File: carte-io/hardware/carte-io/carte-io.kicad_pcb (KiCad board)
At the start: 4 copper layers, 117.5 x 88.5 mm, 193 parts, among them J1 USB_C_Receptacle_USB2.0_14P, J10 JST_PH_B4B, J11 JST_PH_B4B, J12 JST_PH_B4B, J13 JST_PH_B4B, J14 JST_PH_B4B, J15 JST_PH_B4B, J16 JST_PH_B4B, J17 JST_PH_B4B, J18 JST_PH_B4B, J19 JST_PH_B4B, J2 JST-XH_S2B-XH-A, J20 Conn_02x08_Odd_Even, J22 JST_PH_B6B, J23 JST_PH_B4B, J24 JST_PH_B4B, J25 JST_PH_B4B, J26 JST-PH-B2B, J27 JST_PH_B5B, J3 FTSH-105-01-L-DV-007, J4 JST_PH_B4B, J5 JST_PH_B4B, J6 JST_PH_B4B, J7 JST_PH_B4B, J8 TSW-104-07-G-T, J9 TSW-104-07-G-T, SW1 SW_Push, SW2 SW_Push, U1 STM32U545VETx, U10 CM1293A-04SO, U11 74LVC125APW, U12 LSM6DS3, U13 LIS2MDL, U14 LPS22DF, U15 PCA9544APW, U16 LT1963AxST-3.3, U17 PCA9544APW, U18 APDS-9251-001, U19 SHT4x, U2 FT231XQ, U20 74LVC2G125DP,125, U21 CM1293A-04SO, U22 CM1293A-04SO, U23 74LVC125APW, U24 CM1293A-04SO, U25 74LVC125APW, U26 74LVC2G125DP,125, U27 CM1293A-04SO, U28 74LVC2G125DP,125, U29 CM1293A-04SO, U3 LT1963AxST-3.3, U30 74LVC125APW,118, U31 CM1293A-04SO, U32 74LVC2G125DP,125, U33 MCP2542FDxMF, U34 CM1293A-04SO, U35 TCA9802, U36 TPS259250DRCT, U4 CM1293A-04SO, U5 TXU0104PWR, U6 74LVC125APW, U7 CM1293A-04SO, U8 CM1293A-04SO, U9 TXU0104PWR, X1 ASE-16.000MHZ-LC-T

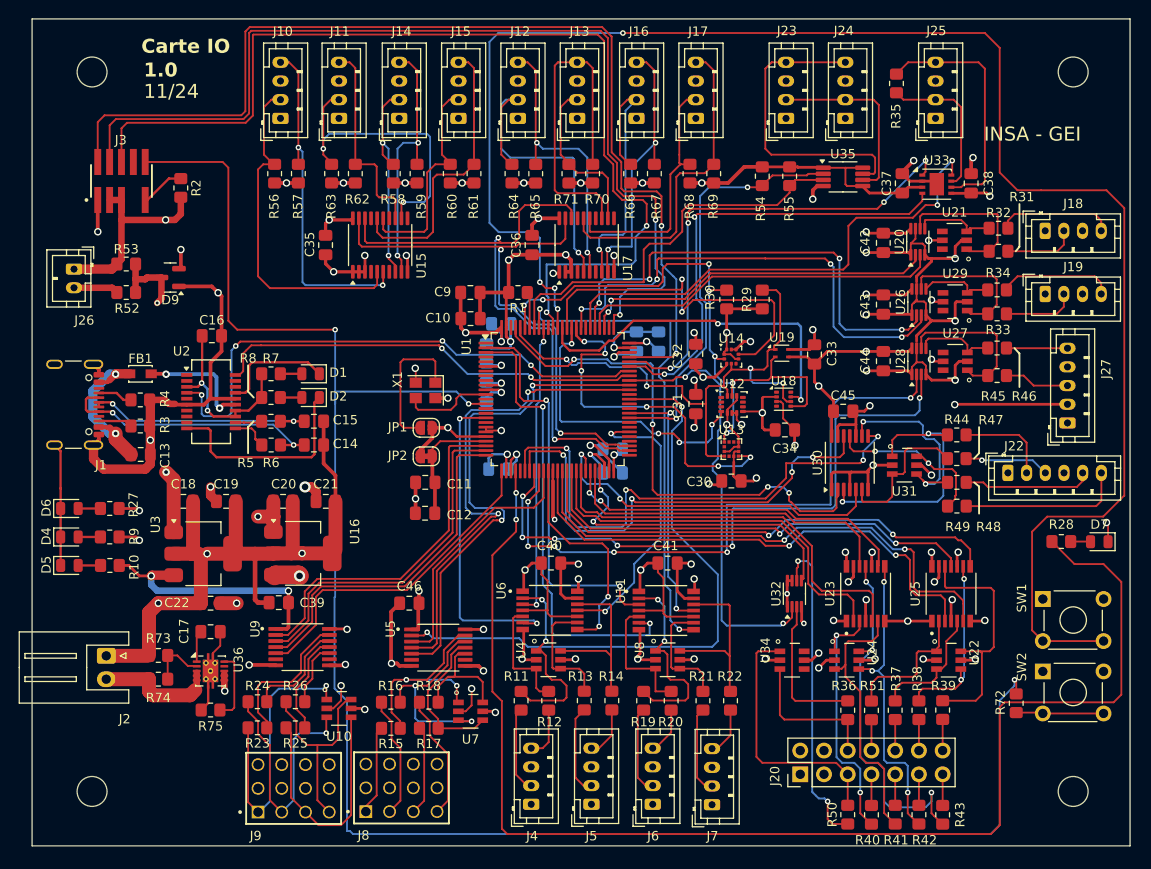
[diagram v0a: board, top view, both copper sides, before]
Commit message: Carte version 1.1 terminée
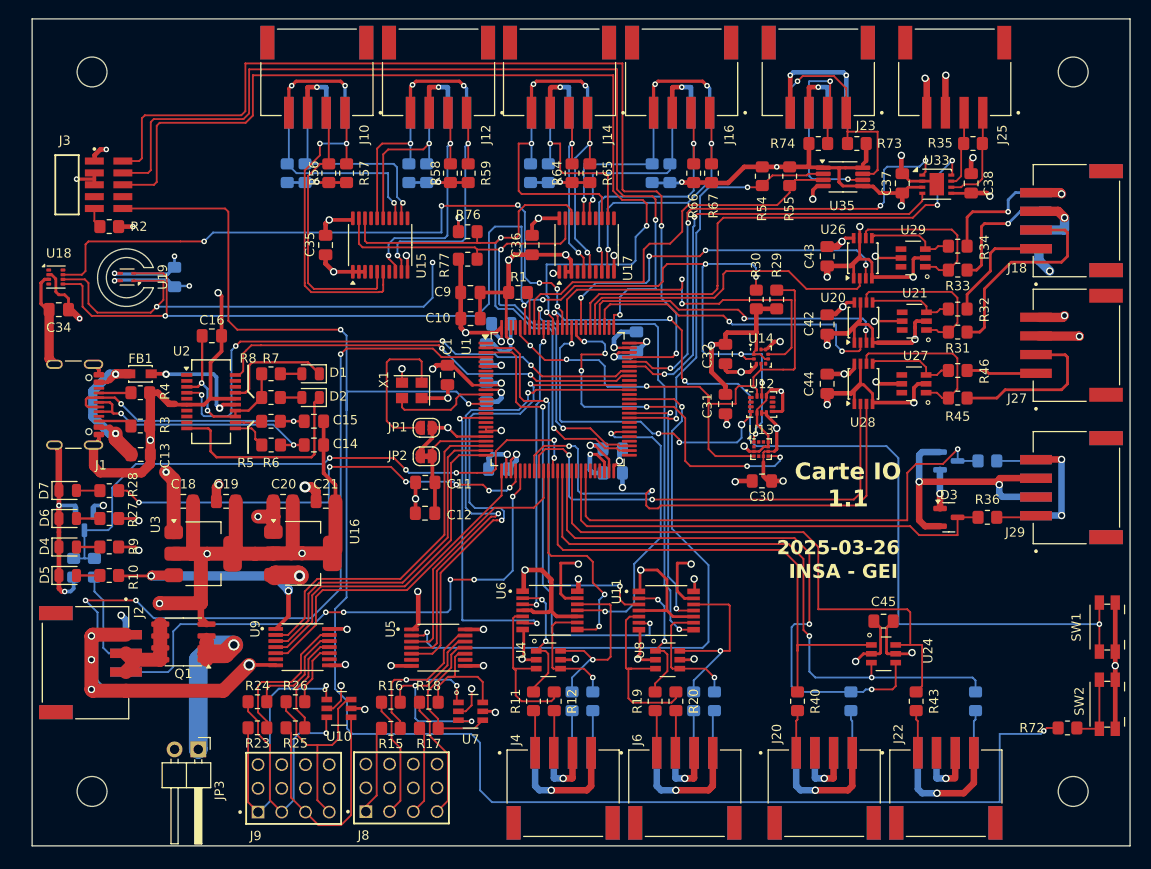
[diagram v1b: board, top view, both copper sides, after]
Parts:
- removed C17: 10µF, Capacitor_SMD:C_0805_2012Metric_Pad1.18x1.45mm_HandSolder
- removed C22, C39, C40, C41, C46: 100nF, Capacitor_SMD:C_0805_2012Metric_Pad1.18x1.45mm_HandSolder
- removed R38, R39, R44, R47, R48, R49, R50, R51: 100R, Resistor_SMD:R_0805_2012Metric_Pad1.20x1.40mm_HandSolder
- removed R75: 5.1K, Resistor_SMD:R_0805_2012Metric_Pad1.20x1.40mm_HandSolder
- removed U22, U31, U34: CM1293A-04SO, CM1293A-04SO:SOT95P285X140-6N
- removed U23, U25: 74LVC125APW, 74LVC125APW:IC_74LVC125APW
- removed U30: 74LVC125APW,118, Package_SO:TSSOP-14_4.4x5mm_P0.65mm
- removed U32: 74LVC2G125DP,125, Package_SO:VSSOP-8_2.3x2mm_P0.5mm
- removed U36: TPS259250DRCT, Package_SON:VSON-10-1EP_3x3mm_P0.5mm_EP1.65x2.4mm_ThermalVias
- added D3: BAT54SFILMY, Package_TO_SOT_SMD:SOT-23, F.Cu at (185.7, 108.7)
- added D8: BAT54SFILMY, Package_TO_SOT_SMD:SOT-23, B.Cu at (185.7, 102.6)
- added J21: 114020164, SeeedStudio - Horizontal Header -114020164:SEEEDSTUDIO_114020164, B.Cu at (172.4, 138.2)
- added J28: 114020164, SeeedStudio - Horizontal Header -114020164:SEEEDSTUDIO_114020164, B.Cu at (185.4, 138.2)
- added J29: 114020164, SeeedStudio - Horizontal Header -114020164:SEEEDSTUDIO_114020164, F.Cu at (199.3, 105.5)
- added J30: 114020164, SeeedStudio - Horizontal Header -114020164:SEEEDSTUDIO_114020164, B.Cu at (199.3, 105.5)
- added JP3: Jumper_2_Bridged, Connector_PinHeader_2.54mm:PinHeader_1x02_P2.54mm_Horizontal, F.Cu at (105.4, 133.5)
- added Q1: IRF9388TRPBF, Package_SO:SOIC-8_3.9x4.9mm_P1.27mm, F.Cu at (103.8, 122.0)
- added R76: 4.7K, Resistor_SMD:R_0805_2012Metric_Pad1.20x1.40mm_HandSolder, F.Cu at (134.2, 78.1)
- added R77: 4.7K, Resistor_SMD:R_0805_2012Metric_Pad1.20x1.40mm_HandSolder, F.Cu at (134.2, 81.0)
- C1: moved to F.Cu
- C33, D9, R13, R14, R21, R22, R37, R41, R42, R52, R53: moved to B.Cu
- J10, J16, J18, J23, J25, J4, J6: value JST_PH_B4B -> 114020164; footprint Connector_JST:JST_PH_B4B-PH-K_1x04_P2.00mm_Vertical -> SeeedStudio - Horizontal Header -114020164:SEEEDSTUDIO_114020164
- J11, J17, J19, J24, J5, J7: value JST_PH_B4B -> 114020164; footprint Connector_JST:JST_PH_B4B-PH-K_1x04_P2.00mm_Vertical -> SeeedStudio - Horizontal Header -114020164:SEEEDSTUDIO_114020164; moved to B.Cu
- J12: renamed from J14; value JST_PH_B4B -> 114020164; footprint Connector_JST:JST_PH_B4B-PH-K_1x04_P2.00mm_Vertical -> SeeedStudio - Horizontal Header -114020164:SEEEDSTUDIO_114020164
- J13: renamed from J15; value JST_PH_B4B -> 114020164; footprint Connector_JST:JST_PH_B4B-PH-K_1x04_P2.00mm_Vertical -> SeeedStudio - Horizontal Header -114020164:SEEEDSTUDIO_114020164; moved to B.Cu
- J14: renamed from J12; value JST_PH_B4B -> 114020164; footprint Connector_JST:JST_PH_B4B-PH-K_1x04_P2.00mm_Vertical -> SeeedStudio - Horizontal Header -114020164:SEEEDSTUDIO_114020164
- J15: renamed from J13; value JST_PH_B4B -> 114020164; footprint Connector_JST:JST_PH_B4B-PH-K_1x04_P2.00mm_Vertical -> SeeedStudio - Horizontal Header -114020164:SEEEDSTUDIO_114020164; moved to B.Cu
- J2: value JST-XH_S2B-XH-A -> 114020164; footprint Connector_JST:JST_XH_S2B-XH-A_1x02_P2.50mm_Horizontal -> SeeedStudio - Horizontal Header -114020164:SEEEDSTUDIO_114020164
- J20: value Conn_02x08_Odd_Even -> 114020164; footprint Connector_PinHeader_2.54mm:PinHeader_2x07_P2.54mm_Vertical -> SeeedStudio - Horizontal Header -114020164:SEEEDSTUDIO_114020164
- J22: value JST_PH_B6B -> 114020164; footprint Connector_JST:JST_PH_B6B-PH-K_1x06_P2.00mm_Vertical -> SeeedStudio - Horizontal Header -114020164:SEEEDSTUDIO_114020164
- J26: value JST-PH-B2B -> 114020164; footprint Connector_JST:JST_PH_B2B-PH-K_1x02_P2.00mm_Vertical -> SeeedStudio - Horizontal Header -114020164:SEEEDSTUDIO_114020164; moved to B.Cu
- J27: value JST_PH_B5B -> 114020164; footprint Connector_JST:JST_PH_B5B-PH-K_1x05_P2.00mm_Vertical -> SeeedStudio - Horizontal Header -114020164:SEEEDSTUDIO_114020164
- J3: value FTSH-105-01-L-DV-007 -> FTSH-105-01-L-DH; footprint FTSH-105-01-L-DV-007-K:SAMTEC_FTSH-105-X-X-DV-007-P-X -> FTSH-105-01-L-DH:SAMTEC_FTSH-105-01-L-DH
- R10, R27: value 100R -> 150R
- R28: value 1K -> 270R
- R29, R30, R54, R55, R56, R57, R58, R59, R64, R65, R66, R67: value 1K -> 4.7K
- R60, R61, R62, R63, R68, R69, R70, R71: value 1K -> 4.7K; moved to B.Cu
- R7, R8: value 1K -> 150R
- R73, R74: value 5.1K -> 4.7K
- R9: value 100R -> 330R
- SW1, SW2: footprint Button_Switch_THT:SW_TH_Tactile_Omron_B3F-10xx -> Button_Switch_SMD:Panasonic_EVQPUJ_EVQPUA
- U20, U26, U28: footprint Package_SO:VSSOP-8_2.3x2mm_P0.5mm -> Package_SO:TSSOP-8_3x3mm_P0.65mm
- moved D7 110.5 mm to (91.4, 105.8), turned to 0 degrees
- moved R28 102.0 mm to (95.8, 105.8), turned to 180 degrees
- moved R73 94.2 mm to (175.8, 68.7), turned to 180 degrees
- moved R74 89.4 mm to (171.7, 68.7), turned to 0 degrees
- moved U18 79.0 mm to (90.1, 82.9)
- moved C34 78.8 mm to (90.4, 86.4), turned to 180 degrees
- moved U19 70.6 mm to (97.7, 82.9), turned to 180 degrees
- moved C33 69.0 mm to (102.8, 82.9), turned to -90 degrees
- moved J26 42.1 mm to (93.3, 124.2), turned to 90 degrees
- moved J22 34.9 mm to (185.4, 138.2)
- moved R53 33.0 mm to (92.0, 114.1), turned to -90 degrees
- moved R52 29.7 mm to (94.2, 114.1), turned to 90 degrees
- moved R37 28.4 mm to (189.8, 102.6), turned to 180 degrees
- moved D9 27.7 mm to (93.2, 109.1), turned to -90 degrees
- moved R36 24.1 mm to (189.8, 108.7), turned to 180 degrees
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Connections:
- J1 pad A6: /Power & Analog/USB-DN -> /Power & Analog/USB-DP
- J1 pad B7: /Power & Analog/USB-DP -> /Power & Analog/USB-DN
- J10 pad 1: +3.3V_PWR -> Net-(J10-Pin_1)
- J10 pad 3: GND -> +3.3V_PWR
- J10 pad 4: Net-(J10-Pin_4) -> GND
- J11 pad 1: +3.3V_PWR -> Net-(J11-Pin_1)
- J11 pad 3: GND -> +3.3V_PWR
- J11 pad 4: Net-(J11-Pin_4) -> GND
- J12 pad 1: +3.3V_PWR -> Net-(J12-Pin_1)
- J12 pad 3: GND -> +3.3V_PWR
- J12 pad 4: Net-(J14-Pin_4) -> GND
- J13 pad 1: +3.3V_PWR -> Net-(J13-Pin_1)
- J13 pad 3: GND -> +3.3V_PWR
- J13 pad 4: Net-(J15-Pin_4) -> GND
- J14 pad 1: +3.3V_PWR -> Net-(J14-Pin_1)
- J14 pad 3: GND -> +3.3V_PWR
- J14 pad 4: Net-(J12-Pin_4) -> GND
- J15 pad 1: +3.3V_PWR -> Net-(J15-Pin_1)
- J15 pad 3: GND -> +3.3V_PWR
- J15 pad 4: Net-(J13-Pin_4) -> GND
- J16 pad 1: +3.3V_PWR -> Net-(J16-Pin_1)
- J16 pad 3: GND -> +3.3V_PWR
- J16 pad 4: Net-(J16-Pin_4) -> GND
- J17 pad 1: +3.3V_PWR -> Net-(J17-Pin_1)
- J17 pad 3: GND -> +3.3V_PWR
- J17 pad 4: Net-(J17-Pin_4) -> GND
- J18 pad 1: +5V -> Net-(J18-Pin_1)
- J18 pad 3: GND -> +5V
- J18 pad 4: Net-(J18-Pin_4) -> GND
- J19 pad 1: +5V -> Net-(J19-Pin_1)
- J19 pad 3: GND -> +5V
- J19 pad 4: Net-(J19-Pin_4) -> GND
- J20 pad 1: +3.3V_PWR -> /GPIO SPI GEN_PWM/IO1
- J20 pad 2: +5V -> unconnected-(J20-Pin_2-Pad2)
- J20 pad 3: GND -> +3.3V
- J22 pad 1: +3.3V_PWR -> /GPIO SPI GEN_PWM/IO4
- J22 pad 2: /GPIO SPI GEN_PWM/SPI_CS_EXT -> unconnected-(J22-Pin_2-Pad2)
- J22 pad 3: /GPIO SPI GEN_PWM/SPI_CLK_EXT -> +3.3V
- J23 pad 1: +3.3V_PWR -> Net-(J23-Pin_1)
- J23 pad 3: GND -> +3.3V_PWR
- J23 pad 4: Net-(J23-Pin_4) -> GND
- J24 pad 1: +3.3V_PWR -> Net-(J23-Pin_1)
- J24 pad 3: GND -> +3.3V_PWR
- J24 pad 4: Net-(J23-Pin_4) -> GND
- J25 pad 1: +5V -> Net-(J25-Pin_1)
- J25 pad 3: GND -> +5V
- J25 pad 4: Net-(J25-Pin_4) -> GND
- J26 pad 1: GND -> /CPU/~{POWEROFF}
- J26 pad 2: Net-(J26-Pin_2) -> /CPU/PWR_CSLEEP
- J27 pad 1: +5V -> Net-(J27-Pin_1)
- J27 pad 2: +3.3V -> Net-(J27-Pin_2)
- J27 pad 3: Net-(J27-Pin_3) -> +5V
- J4 pad 1: +3.3V -> Net-(J4-Pin_1)
- J4 pad 3: GND -> +3.3V
- J4 pad 4: Net-(J4-Pin_4) -> GND
- J5 pad 1: +3.3V -> Net-(J5-Pin_1)
- J5 pad 3: GND -> +3.3V
- J5 pad 4: Net-(J5-Pin_4) -> GND
- J6 pad 1: +3.3V -> Net-(J6-Pin_1)
- J6 pad 3: GND -> +3.3V
- J6 pad 4: Net-(J6-Pin_4) -> GND
- J7 pad 1: +3.3V -> Net-(J7-Pin_1)
- J7 pad 3: GND -> +3.3V
- J7 pad 4: Net-(J7-Pin_4) -> GND
- R11 pad 1: Net-(J4-Pin_2) -> Net-(J4-Pin_1)
- R12 pad 1: Net-(J4-Pin_4) -> Net-(J4-Pin_2)
- R13 pad 1: Net-(J5-Pin_2) -> Net-(J5-Pin_1)
- R14 pad 1: Net-(J5-Pin_4) -> Net-(J5-Pin_2)
- R19 pad 1: Net-(J6-Pin_2) -> Net-(J6-Pin_1)
- R20 pad 1: Net-(J6-Pin_4) -> Net-(J6-Pin_2)
- R21 pad 1: Net-(J7-Pin_2) -> Net-(J7-Pin_1)
- R22 pad 1: Net-(J7-Pin_4) -> Net-(J7-Pin_2)
- R32 pad 2: Net-(J18-Pin_4) -> Net-(J18-Pin_1)
- R34 pad 2: Net-(J19-Pin_4) -> Net-(J19-Pin_1)
- R35 pad 2: Net-(J25-Pin_4) -> Net-(J25-Pin_1)
- R36 pad 1: /GPIO SPI GEN_PWM/IN1 -> /GPIO SPI GEN_PWM/AN1
- R36 pad 2: Net-(U22-CH1) -> /CPU/ADC_AN1
- R37 pad 1: /GPIO SPI GEN_PWM/IN2 -> Net-(J30-Pin_1)
- R37 pad 2: Net-(U22-CH2) -> /CPU/ADC_AN2
- R40 pad 1: Net-(U23-1Y) -> /CPU/IO1
- R40 pad 2: /GPIO SPI GEN_PWM/OUT1 -> /GPIO SPI GEN_PWM/IO1
- R41 pad 1: Net-(U23-2Y) -> /CPU/IO2
- R41 pad 2: /GPIO SPI GEN_PWM/OUT2 -> /GPIO SPI GEN_PWM/IO2
- R42 pad 1: Net-(U23-3Y) -> /CPU/IO3
- R42 pad 2: /GPIO SPI GEN_PWM/OUT3 -> /GPIO SPI GEN_PWM/IO3
- R43 pad 1: Net-(U23-4Y) -> /CPU/IO4
- R43 pad 2: /GPIO SPI GEN_PWM/OUT4 -> /GPIO SPI GEN_PWM/IO4
- R45 pad 2: Net-(J27-Pin_3) -> Net-(J27-Pin_2)
- R46 pad 2: Net-(J27-Pin_5) -> Net-(J27-Pin_1)
- R52 pad 1: Net-(J26-Pin_2) -> Net-(J26-Pin_3)
- R57 pad 2: Net-(J10-Pin_4) -> Net-(J10-Pin_1)
- R59 pad 2: Net-(J14-Pin_4) -> Net-(J12-Pin_1)
- R61 pad 2: Net-(J15-Pin_4) -> Net-(J13-Pin_1)
- R62 pad 1: Net-(J11-Pin_4) -> Net-(J11-Pin_1)
- R65 pad 2: Net-(J12-Pin_4) -> Net-(J14-Pin_1)
- R67 pad 2: Net-(J16-Pin_4) -> Net-(J16-Pin_1)
- R69 pad 2: Net-(J17-Pin_4) -> Net-(J17-Pin_1)
- R70 pad 1: Net-(J13-Pin_4) -> Net-(J15-Pin_1)
- R73 pad 1: /Power & Analog/VIN -> +3.3V
- R73 pad 2: Net-(U36-EN/UVLO) -> Net-(J23-Pin_1)
- R74 pad 1: Net-(U36-EN/UVLO) -> +3.3V
- R74 pad 2: GND -> Net-(J23-Pin_2)
- U1 pad 31: /CPU/SPI_MISO -> unconnected-(U1-PA6-Pad31)
- U1 pad 32: /CPU/SPI_MOSI -> unconnected-(U1-PA7-Pad32)
- U1 pad 38: /CPU/INPUT1 -> /CPU/IO1
- U1 pad 39: /CPU/INPUT2 -> /CPU/IO2
- U1 pad 40: /CPU/INPUT3 -> /CPU/IO3
- U1 pad 41: /CPU/INPUT4 -> /CPU/IO4
- U1 pad 42: /CPU/OUTPUT1 -> unconnected-(U1-PE11-Pad42)
- U1 pad 43: /CPU/OUTPUT2 -> /CPU/ADC_AN1
- U1 pad 44: /CPU/SPI_SCK -> /CPU/ADC_AN2
- U1 pad 45: /CPU/OUTPUT3 -> unconnected-(U1-PE14-Pad45)
- U1 pad 46: /CPU/OUTPUT4 -> unconnected-(U1-PE15-Pad46)
- U1 pad 47: /CPU/GEN_PWM2 -> unconnected-(U1-PB10-Pad47)
- U1 pad 67: /CPU/GEN_PWM1 -> unconnected-(U1-PA8-Pad67)
- U1 pad 97: /CPU/SPI_CS -> unconnected-(U1-PE0-Pad97)
- U15 pad 13: Net-(J11-Pin_4) -> Net-(J11-Pin_1)
- U15 pad 16: Net-(J15-Pin_4) -> Net-(J13-Pin_1)
- U15 pad 6: Net-(J10-Pin_4) -> Net-(J10-Pin_1)
- U15 pad 9: Net-(J14-Pin_4) -> Net-(J12-Pin_1)
- U17 pad 13: Net-(J13-Pin_4) -> Net-(J15-Pin_1)
- U17 pad 16: Net-(J17-Pin_4) -> Net-(J17-Pin_1)
- U17 pad 6: Net-(J12-Pin_4) -> Net-(J14-Pin_1)
- U17 pad 9: Net-(J16-Pin_4) -> Net-(J16-Pin_1)
- U21 pad 5: +5V -> +3.3V
- U24 pad 1: Net-(U23-1Y) -> /CPU/IO1
- U24 pad 3: Net-(U23-2Y) -> /CPU/IO2
- U24 pad 4: Net-(U23-3Y) -> /CPU/IO3
- U24 pad 6: Net-(U23-4Y) -> /CPU/IO4
- U27 pad 5: +5V -> +3.3V
- U29 pad 5: +5V -> +3.3V
- U33 pad 6: Net-(J25-Pin_4) -> Net-(J25-Pin_1)
- U35 pad 7: Net-(J23-Pin_4) -> Net-(J23-Pin_1)
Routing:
- net GND: track 440.5 -> 556.9 mm, vias 62 -> 78
- net /CPU/LED_ACTIVITY: track 141.2 -> 49.7 mm, vias 2 -> 6
- net /CPU/USER_BTN: track 181.2 -> 95.4 mm
- net /CPU/~{POWEROFF}: track 0.00 -> 83.3 mm, vias 0 -> 3
- net /CPU/I2C_SCL_INT: track 65.7 -> 137.7 mm, vias 7 -> 8
- net /CPU/I2C_SDA_INT: track 63.1 -> 132.4 mm, vias 4 -> 5
- net +3.3V: track 330.3 -> 398.7 mm, vias 51 -> 52
- net /CPU/IO2: track 0.00 -> 67.2 mm, vias 0 -> 2
- net +3.3V_PWR: track 191.9 -> 126.8 mm, vias 3 -> 8
- net /CPU/IO3: track 0.00 -> 63.4 mm, vias 0 -> 2
- net /CPU/IO4: track 0.00 -> 61.2 mm
- net /CPU/PWR_CSLEEP: track 0.00 -> 61.0 mm, vias 0 -> 5
- net /CPU/SPI_MISO: track 57.4 -> 0.00 mm, vias 4 -> 0
- net /CPU/INPUT2: track 56.9 -> 0.00 mm, vias 2 -> 0
- net /CPU/IO1: track 0.00 -> 56.6 mm
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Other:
- outline, holes or cut-outs redrawn
- board text added: "${COMPANY}"
- board text added: "${ISSUE_DATE}"
- board text added: "${TITLE} ${REVISION}"
- board text removed: "1.0"
- board text removed: "11/24"
- board text removed: "Carte IO"
- board text removed: "INSA - GEI"
